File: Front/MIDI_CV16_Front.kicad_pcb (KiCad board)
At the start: 2 copper layers, 59.5 x 128.5 mm, 23 parts, among them J1 Screw_Terminal_01x01, J10 Conn_01x01, J11 Conn_01x01, J12 Conn_01x01, J13 Conn_01x01, J14 Conn_01x01, J15 Conn_01x01, J16 Conn_01x01, J17 Conn_01x01, J18 Conn_01x01, J19 Conn_01x01, J2 Screw_Terminal_01x01, J20 Conn_01x01, J21 Conn_01x01, J22 Conn_01x01, J23 Conn_01x01, J3 Screw_Terminal_01x01, J4 Screw_Terminal_01x01, J5 Conn_01x01, J6 Conn_01x01, J7 Conn_01x01, J8 Conn_01x01, J9 Conn_01x01

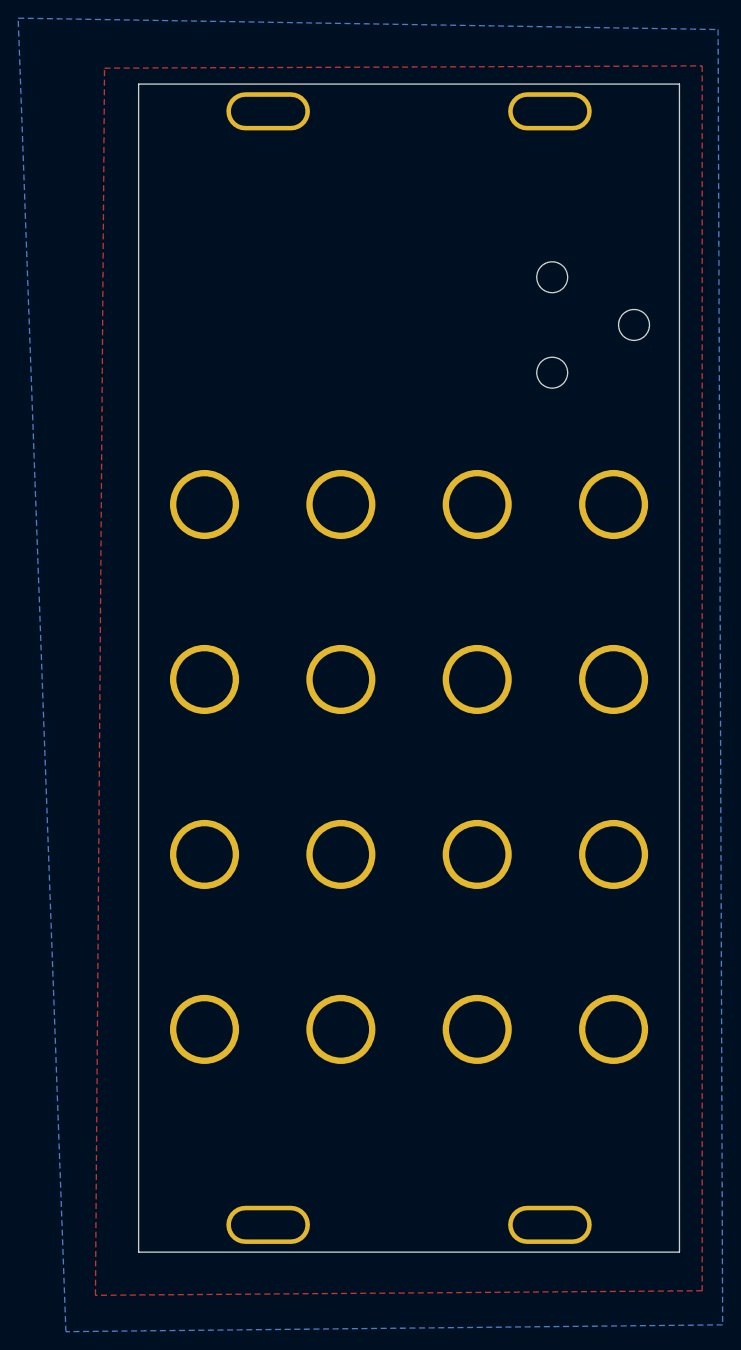
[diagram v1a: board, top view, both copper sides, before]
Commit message: Finalize module
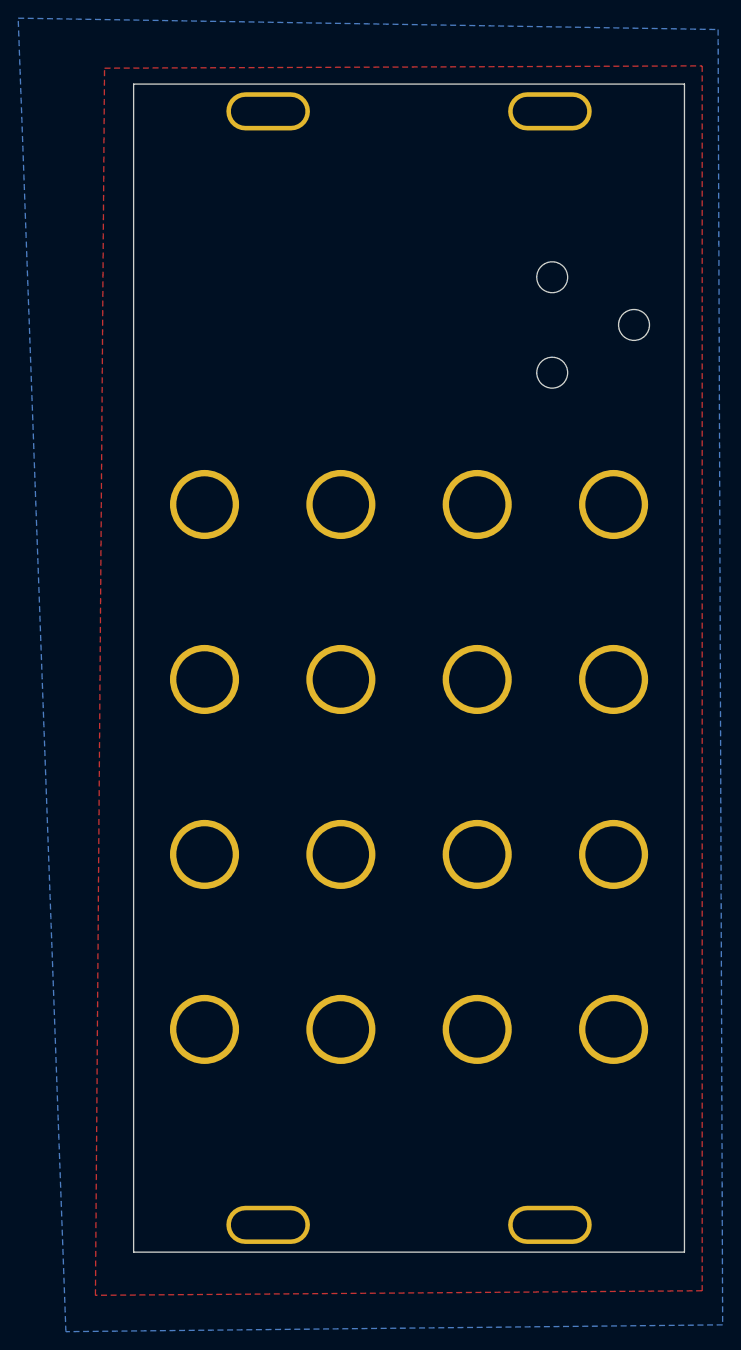
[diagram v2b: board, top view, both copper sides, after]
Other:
- board size 59.5 x 128.5 mm -> 60.6 x 128.5 mm
- rule pad_to_mask_clearance: 0.05 -> 0
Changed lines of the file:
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@@
   )
   (setup
-    (pad_to_mask_clearance 0.05)
+    (pad_to_mask_clearance 0)
     (pcbplotparams
       (layerselection 0x00010f0_ffffffff)
@@
       (psnegative false)
       (psa4output false)
-      (plotreference true)
+      (plotreference false)
       (plotvalue false)
       (plotinvisibletext false)
@@
       (drillshape 0)
       (scaleselection 1)
-      (outputdirectory "Gerbers/Front/")
+      (outputdirectory "outputs/")
     )
   )
@@
   (gr_line (start 67.75 72.5) (end 67.75 51.25)
     (stroke (width 0.15) (type solid)) (layer "Dwgs.User"))
-  (gr_line (start 50.25 35.5) (end 50.25 164)
+  (gr_line (start 49.7 35.5) (end 49.7 164)
     (stroke (width 0.05) (type solid)) (layer "Edge.Cuts"))
-  (gr_line (start 109.75 35.5) (end 50.25 35.5)
+  (gr_line (start 110.3 35.5) (end 49.7 35.5)
     (stroke (width 0.05) (type solid)) (layer "Edge.Cuts"))
-  (gr_line (start 109.75 164) (end 109.75 35.5)
+  (gr_line (start 110.3 164) (end 110.3 35.5)
     (stroke (width 0.05) (type solid)) (layer "Edge.Cuts"))
-  (gr_line (start 50.25 164) (end 109.75 164)
+  (gr_line (start 49.7 164) (end 110.3 164)
     (stroke (width 0.05) (type solid)) (layer "Edge.Cuts"))
   (gr_text "JLCJLCJLCJLC" (at 80 154) (layer "B.SilkS")
